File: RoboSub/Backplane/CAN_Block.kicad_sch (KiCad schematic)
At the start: 3 parts, among them U3 TCAN330G

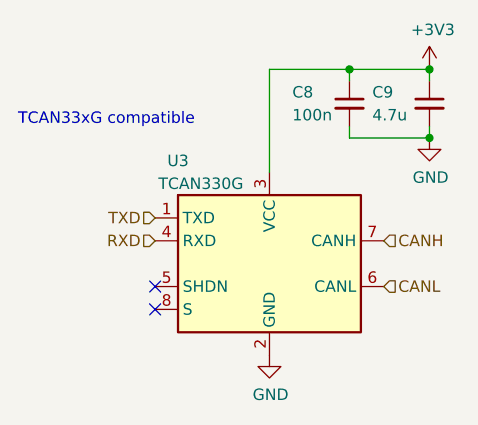
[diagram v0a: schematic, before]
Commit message: add libs
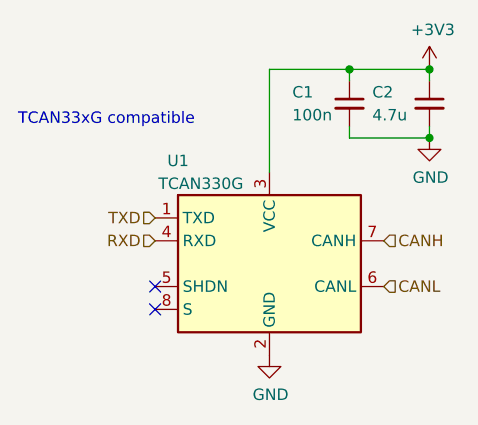
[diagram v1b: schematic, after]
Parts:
- renumbered C8 to C1, C9 to C2, U3 to U1
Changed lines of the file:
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@@
   (symbol (lib_id "power:GND") (at 152.4 83.82 0)
     (in_bom yes) (on_board yes)
-    (property "Reference" "#PWR041" (id 0) (at 152.4 90.17 0)
+    (property "Reference" "#PWR032" (id 0) (at 152.4 90.17 0)
       (effects (font (size 1.27 1.27)) hide)
     )
@@
   (symbol (lib_id "power:+3V3") (at 152.4 76.2 0)
     (in_bom yes) (on_board yes)
-    (property "Reference" "#PWR040" (id 0) (at 152.4 80.01 0)
+    (property "Reference" "#PWR031" (id 0) (at 152.4 80.01 0)
       (effects (font (size 1.27 1.27)) hide)
     )
@@
   (symbol (lib_id "power:GND") (at 134.62 107.95 0)
     (in_bom yes) (on_board yes)
-    (property "Reference" "#PWR039" (id 0) (at 134.62 114.3 0)
+    (property "Reference" "#PWR030" (id 0) (at 134.62 114.3 0)
       (effects (font (size 1.27 1.27)) hide)
     )
@@
   (symbol (lib_id "Device:C_Small") (at 152.4 80.01 0)
     (in_bom yes) (on_board yes)
-    (property "Reference" "C9" (id 0) (at 146.05 78.74 0)
+    (property "Reference" "C2" (id 0) (at 146.05 78.74 0)
       (effects (font (size 1.27 1.27)) (justify left))
     )
@@
   (symbol (lib_id "Device:C_Small") (at 143.51 80.01 0)
     (in_bom yes) (on_board yes)
-    (property "Reference" "C8" (id 0) (at 137.16 78.74 0)
+    (property "Reference" "C1" (id 0) (at 137.16 78.74 0)
       (effects (font (size 1.27 1.27)) (justify left))
     )
@@
   (symbol (lib_id "Interface_CAN_LIN:TCAN330G") (at 134.62 97.79 0)
     (in_bom yes) (on_board yes)
-    (property "Reference" "U3" (id 0) (at 124.46 86.36 0))
+    (property "Reference" "U1" (id 0) (at 124.46 86.36 0))
     (property "Value" "TCAN330G" (id 1) (at 127 88.9 0))
     (property "Footprint" "Package_SO:SOIC-8_3.9x4.9mm_P1.27mm" (id 2) (at 134.62 110.49 0)
